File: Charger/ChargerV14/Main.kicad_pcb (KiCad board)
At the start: 2 copper layers, 25.4 x 27.8 mm, 25 parts, among them J1 TX_Coil, J6 Coil B, J8 USB_C_Receptacle_USB2.0, J9 Coil A, U2 XKT335, U3 XKT001

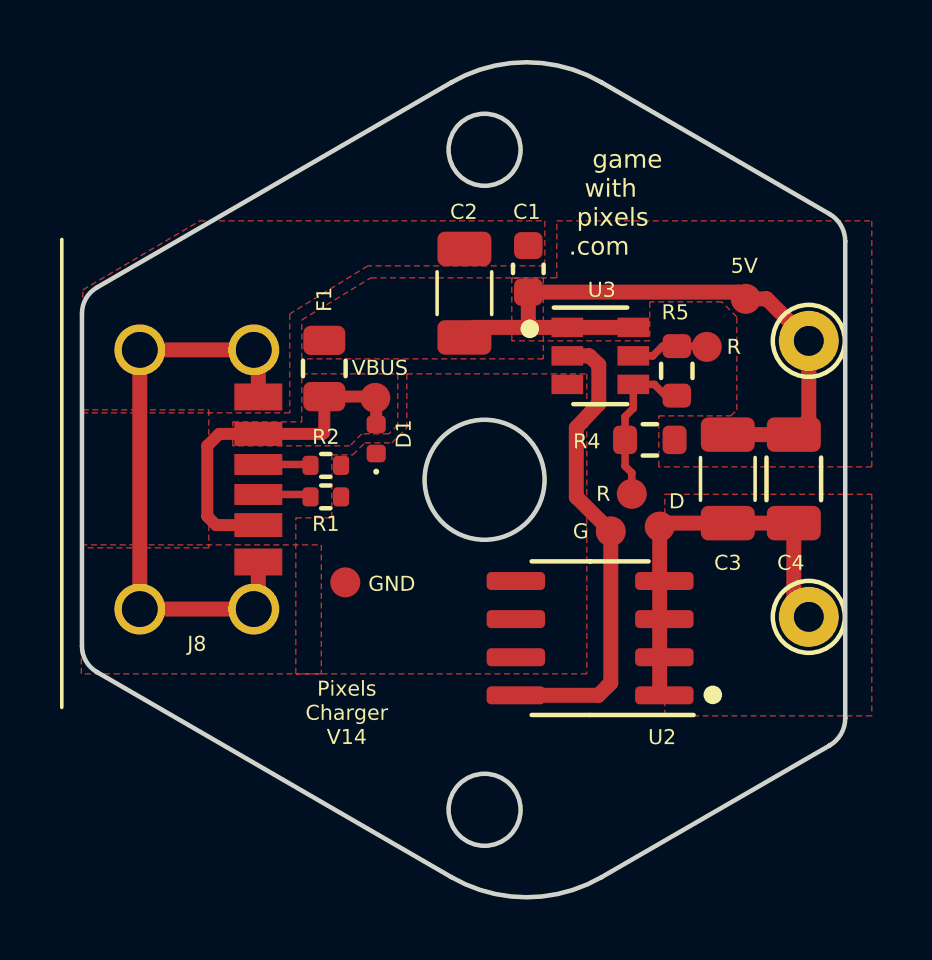
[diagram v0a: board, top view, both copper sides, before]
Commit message: Single Charger V14
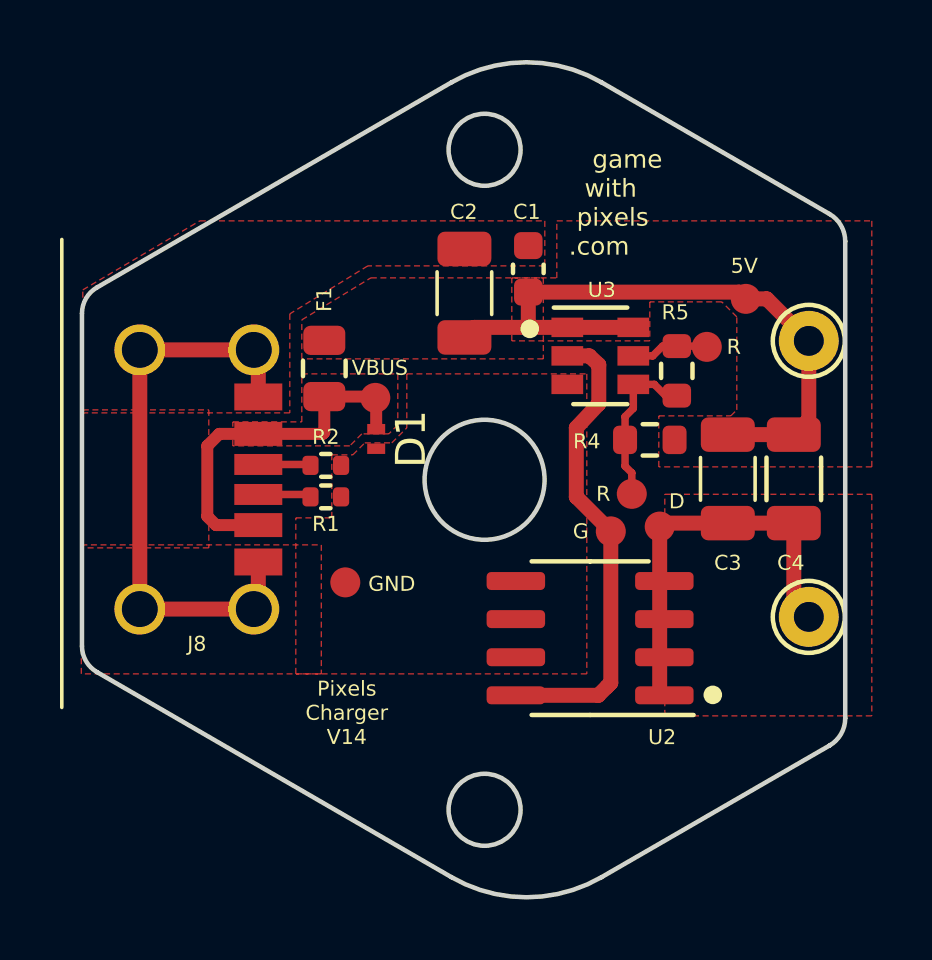
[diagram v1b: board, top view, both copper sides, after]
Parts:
- D1: footprint Diode_SMD:D_0402_1005Metric -> Pixels-dice:DFN
- turned D1 to -90 degrees
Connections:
- D1 pad 1: GND -> VBUS
- D1 pad 2: VBUS -> GND
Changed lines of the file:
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@@
       (net 5 "Net-(U2-Pad8)") (pinfunction "1") (pintype "passive"))
   )
-  (footprint "Diode_SMD:D_0402_1005Metric" (layer "F.Cu")
-    (at 146.28 100.17 90)
-    (descr "Diode SMD 0402 (1005 Metric), square (rectangular) end terminal, IPC_7351 nominal, (Body size source: http://www.tortai-tech.com/upload/download/2011102023233369053.pdf), generated with kicad-footprint-generator")
-    (tags "diode")
+  (footprint "Pixels-dice:DFN" (layer "F.Cu")
+    (at 146.28 100.17 -90)
+    (descr "Capacitor SMD 0402 (1005 Metric), square (rectangular) end terminal, IPC_7351 nominal, (Body size source: IPC-SM-782 page 76, https://www.pcb-3d.com/wordpress/wp-content/uploads/ipc-sm-782a_amendment_1_and_2.pdf), generated with kicad-footprint-generator")
+    (tags "capacitor")
     (property "Manufacturer" "Murata")
     (property "Part Number" "LXES1UTAA1-157")
@@
     (property "Sheetname" "")
     (attr smd)
-    (fp_text reference "D1" (at 0.17 0.92 90) (layer "F.SilkS")
-      (effects (font (size 0.5 0.5) (thickness 0.12)))
+    (fp_text reference "D1" (at 0 -1.16 90) (layer "F.SilkS")
+      (effects (font (size 1 1) (thickness 0.15)))
     )
-    (fp_text value "D_TVS" (at 0 1.17 90) (layer "F.Fab")
-      (effects (font (size 0.5 0.5) (thickness 0.12)))
+    (fp_text value "D_TVS" (at 0 1.16 90) (layer "F.Fab")
+      (effects (font (size 1 1) (thickness 0.15)))
     )
-    (fp_text user "${REFERENCE}" (at 0 0 90) (layer "F.Fab")
+    (fp_text user "${REFERENCE}" (at 0 -0.5 90) (layer "F.Fab")
       (effects (font (size 0.25 0.25) (thickness 0.04)))
     )
-    (fp_circle (center -1.09 0) (end -1.04 0) (layer "F.SilkS") (width 0.1) (fill none))
-    (fp_line (start 0.93 0.47) (end -0.93 0.47) (layer "F.CrtYd") (width 0.05))
-    (fp_line (start 0.93 -0.47) (end 0.93 0.47) (layer "F.CrtYd") (width 0.05))
-    (fp_line (start -0.93 0.47) (end -0.93 -0.47) (layer "F.CrtYd") (width 0.05))
-    (fp_line (start -0.93 -0.47) (end 0.93 -0.47) (layer "F.CrtYd") (width 0.05))
-    (fp_line (start -0.4 0.25) (end -0.4 -0.25) (layer "F.Fab") (width 0.1))
-    (fp_line (start -0.3 0.25) (end -0.3 -0.25) (layer "F.Fab") (width 0.1))
-    (fp_line (start -0.5 -0.25) (end 0.5 -0.25) (layer "F.Fab") (width 0.1))
-    (fp_line (start -0.5 0.25) (end -0.5 -0.25) (layer "F.Fab") (width 0.1))
-    (fp_line (start 0.5 -0.25) (end 0.5 0.25) (layer "F.Fab") (width 0.1))
-    (fp_line (start 0.5 0.25) (end -0.5 0.25) (layer "F.Fab") (width 0.1))
-    (pad "1" smd roundrect (at -0.485 0 90) (size 0.59 0.64) (layers "F.Cu" "F.Paste" "F.Mask") (roundrect_rratio 0.25)
-      (net 1 "GND") (pinfunction "A1") (pintype "passive"))
-    (pad "2" smd roundrect (at 0.485 0 90) (size 0.59 0.64) (layers "F.Cu" "F.Paste" "F.Mask") (roundrect_rratio 0.25)
-      (net 2 "VBUS") (pinfunction "A2") (pintype "passive"))
-    (model "${KICAD6_3DMODEL_DIR}/Diode_SMD.3dshapes/D_0402_1005Metric.wrl"
+    (fp_circle (center -0.7 0) (end -0.7 0) (layer "F.SilkS") (width 0.12) (fill none))
+    (fp_line (start -0.91 0.46) (end -0.91 -0.46) (layer "F.CrtYd") (width 0.05))
+    (fp_line (start 0.91 0.46) (end -0.91 0.46) (layer "F.CrtYd") (width 0.05))
+    (fp_line (start -0.91 -0.46) (end 0.91 -0.46) (layer "F.CrtYd") (width 0.05))
+    (fp_line (start 0.91 -0.46) (end 0.91 0.46) (layer "F.CrtYd") (width 0.05))
+    (fp_line (start -0.4 0.25) (end -0.4 -0.25) (layer "F.Fab") (width 0.05))
+    (fp_line (start 0.4 0.25) (end -0.4 0.25) (layer "F.Fab") (width 0.05))
+    (fp_line (start -0.4 -0.25) (end 0.4 -0.25) (layer "F.Fab") (width 0.05))
+    (fp_line (start 0.4 -0.25) (end 0.4 0.25) (layer "F.Fab") (width 0.05))
+    (pad "1" smd rect (at -0.325 0 270) (size 0.35 0.6) (layers "F.Cu" "F.Paste" "F.Mask")
+      (net 2 "VBUS") (pinfunction "A1") (pintype "passive"))
+    (pad "2" smd rect (at 0.325 0 270) (size 0.35 0.6) (layers "F.Cu" "F.Paste" "F.Mask")
+      (net 1 "GND") (pinfunction "A2") (pintype "passive"))
+    (model "${KICAD6_3DMODEL_DIR}/Capacitor_SMD.3dshapes/C_0402_1005Metric.wrl"
       (offset (xyz 0 0 0))
       (scale (xyz 1 1 1))
